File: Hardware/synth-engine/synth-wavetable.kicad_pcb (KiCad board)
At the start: 2 copper layers, 100 x 100 mm, 152 parts, among them J1 SWD_programming, J2 USB-B-S, J3 MIDI_IN, J4 MIDI_OUT, J5 SWD_JTAG, J6 AUDIO-JACK4-.25-HORIZ-TRS, J7 POWER_JACKPTH, J8 Conn_02x12_Odd_Even, Q1 2N3904, U1 CY8C4246AZI-L445, U10 NJM4580, U3 STM32F429VETx, U4 TL074CN, U5 SSI2144, U6 V7805-1000, U7 XC6219-3.3, U8 XC6219-3.3, U9 AK4490, Y1 16MHz, Y2 16MHz

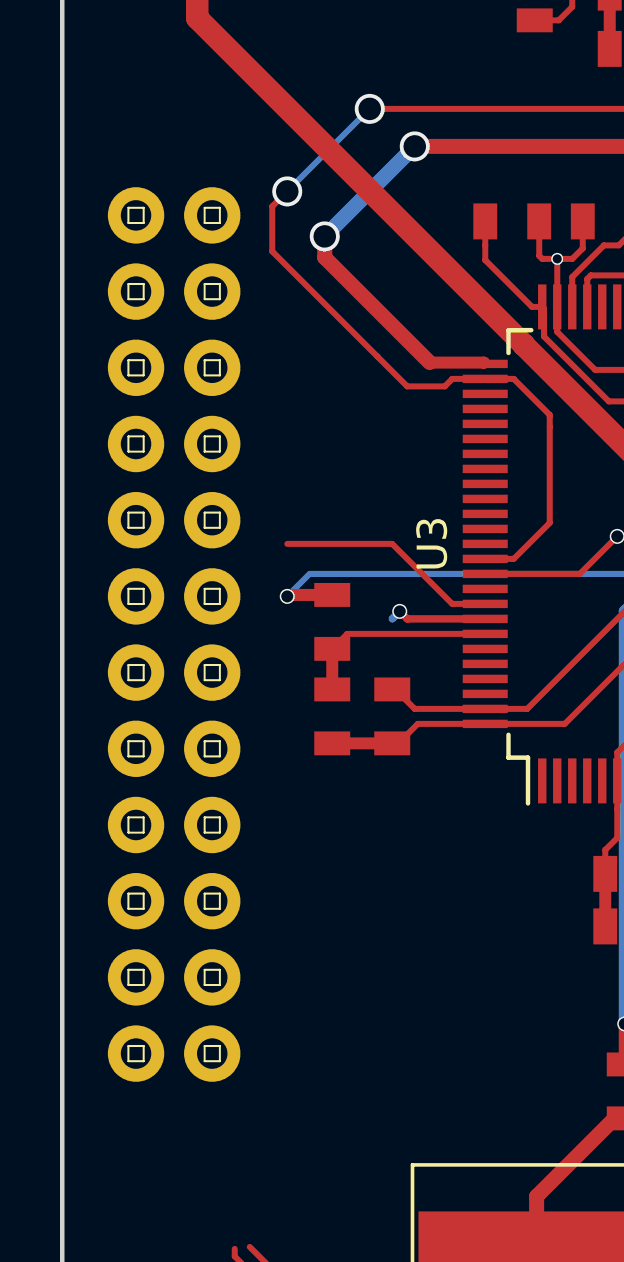
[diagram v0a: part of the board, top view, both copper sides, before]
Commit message: route control board
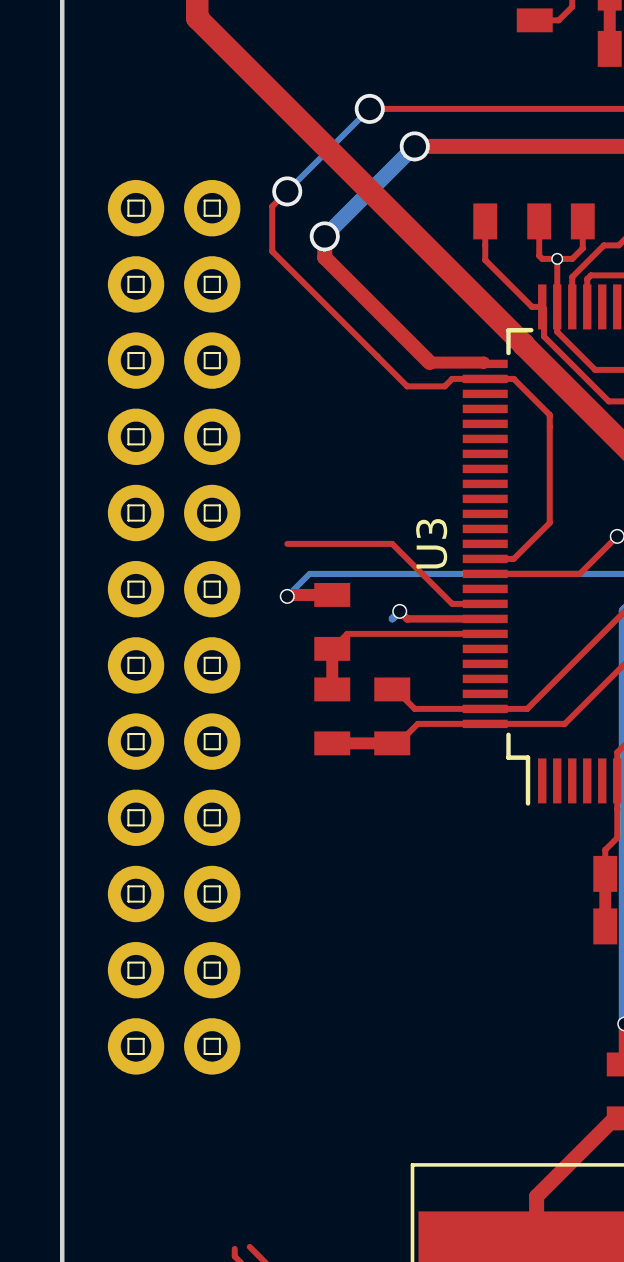
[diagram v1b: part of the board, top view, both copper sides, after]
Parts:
- moved J8 0.24 mm to (3.73, 74.0)
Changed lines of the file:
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@@
   )
   (module SparkFun-Connectors:2X12 (layer F.Cu)
-    (at 3.73 74.27 90)
+    (at 3.73 74.03 90)
     (attr virtual)
     (fp_text reference J8 (at -12.065 -3.81 90) (layer B.SilkS)
